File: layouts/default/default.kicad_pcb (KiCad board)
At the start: 2 copper layers, 28.8 x 41.5 mm, 46 parts

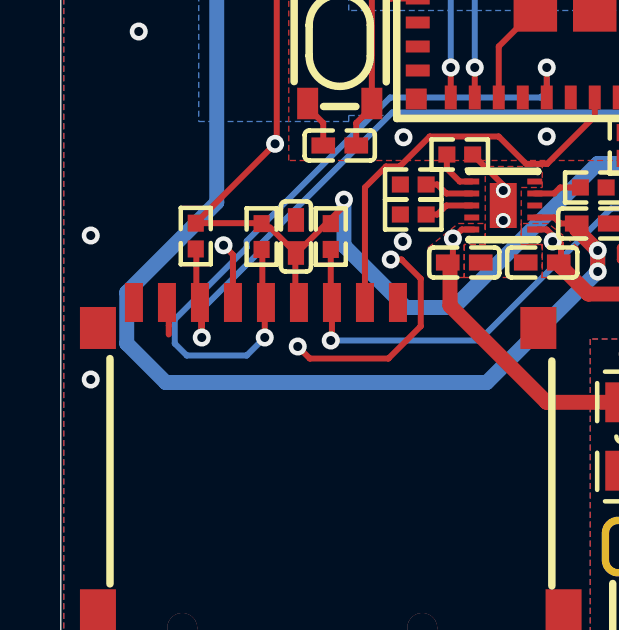
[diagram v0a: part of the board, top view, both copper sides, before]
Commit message: cleaning up readme
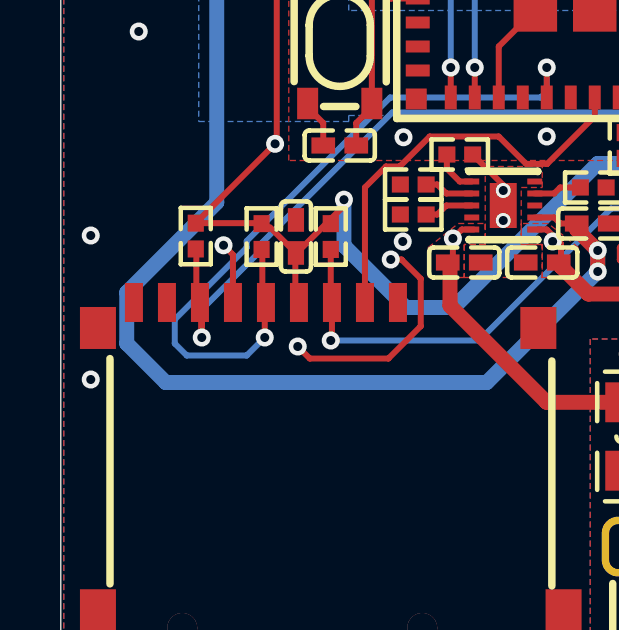
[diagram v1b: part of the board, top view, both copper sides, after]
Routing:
- net DAT1: track 1.30 -> 0.00 mm
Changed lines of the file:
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@@
 			(layer "F.Fab")
 		)
-		(fp_text user "${REFERENCE}"
-			(at 0 0 180)
-			(layer "F.Fab")
-			(effects
-				(font
-					(size 1 1)
-					(thickness 0.15)
-				)
-			)
-		)
 		(pad "1" smd rect
 			(at -0.55 0 180)
@@
 			(layer "F.Fab")
 		)
-		(fp_text user "${REFERENCE}"
-			(at 0 0 0)
-			(layer "F.Fab")
-			(effects
-				(font
-					(size 1 1)
-					(thickness 0.15)
-				)
-			)
-		)
 		(pad "1" smd rect
 			(at -0.43 0 270)
@@
 			(layer "F.Fab")
 		)
-		(fp_text user "${REFERENCE}"
-			(at 0 0 0)
-			(layer "F.Fab")
-			(effects
-				(font
-					(size 1 1)
-					(thickness 0.15)
-				)
-			)
-		)
 		(pad "1" smd rect
 			(at -0.43 0 270)
@@
 			(layer "F.Fab")
 		)
-		(fp_text user "${REFERENCE}"
-			(at 0 0 0)
-			(layer "F.Fab")
-			(effects
-				(font
-					(size 1 1)
-					(thickness 0.15)
-				)
-			)
-		)
 		(pad "1" smd rect
 			(at -0.43 0)
@@
 			(layer "F.Fab")
 		)
-		(fp_text user "${REFERENCE}"
-			(at 0 0 0)
-			(layer "F.Fab")
-			(effects
-				(font
-					(size 1 1)
-					(thickness 0.15)
-				)
-			)
-		)
 		(pad "1" smd rect
 			(at 0.65 0.65)
@@
 	)
 	(segment
-		(start 119 102.2)
-		(end 119 102.5)
-		(width 0.2)
-		(layer "F.Cu")
-		(net 30)
-	)
-	(segment
-		(start 119 101.2)
-		(end 119 102.2)
-		(width 0.2)
-		(layer "F.Cu")
-		(net 30)
-	)
-	(segment
